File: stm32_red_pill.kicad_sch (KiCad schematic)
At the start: 29 parts, among them J1 USB_B_Micro, J2 Conn_01x18, J3 Conn_01x18, SW1 SW_SPDT, U1 STM32F103C8T6, U2 AMS1117-3.3, Y1 16MHZ

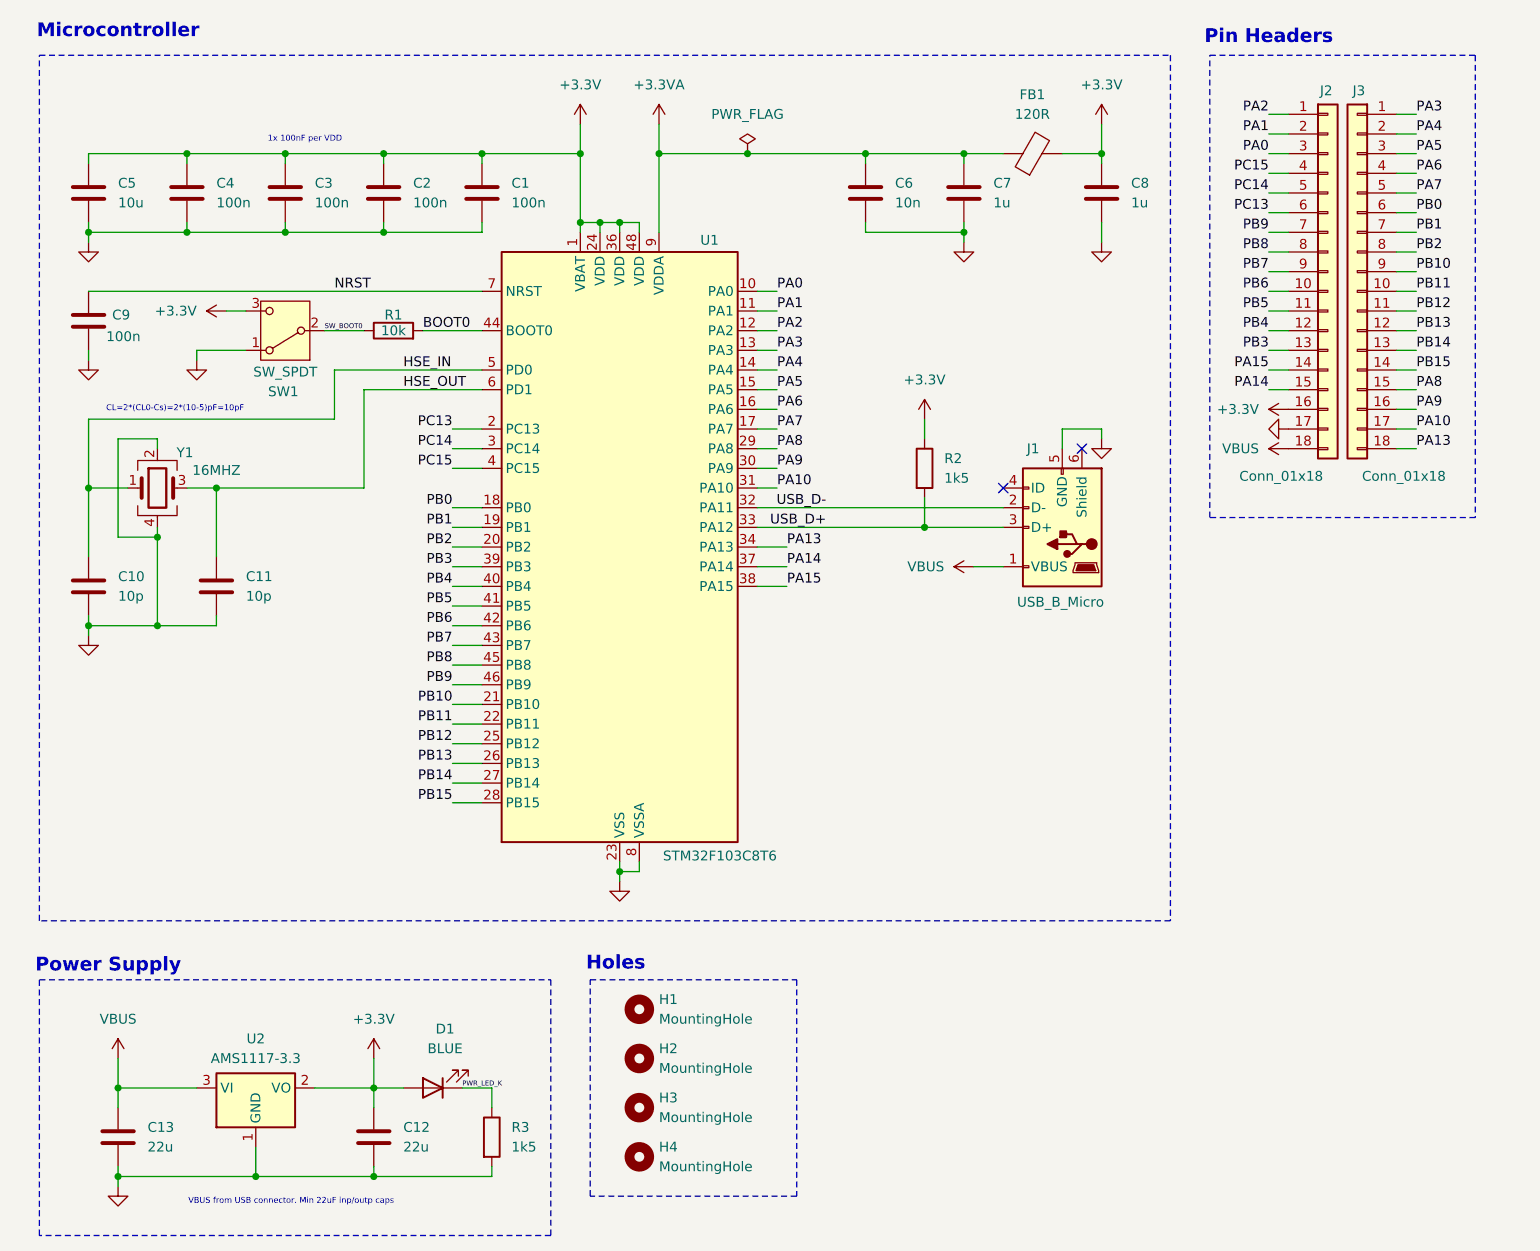
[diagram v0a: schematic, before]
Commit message: update
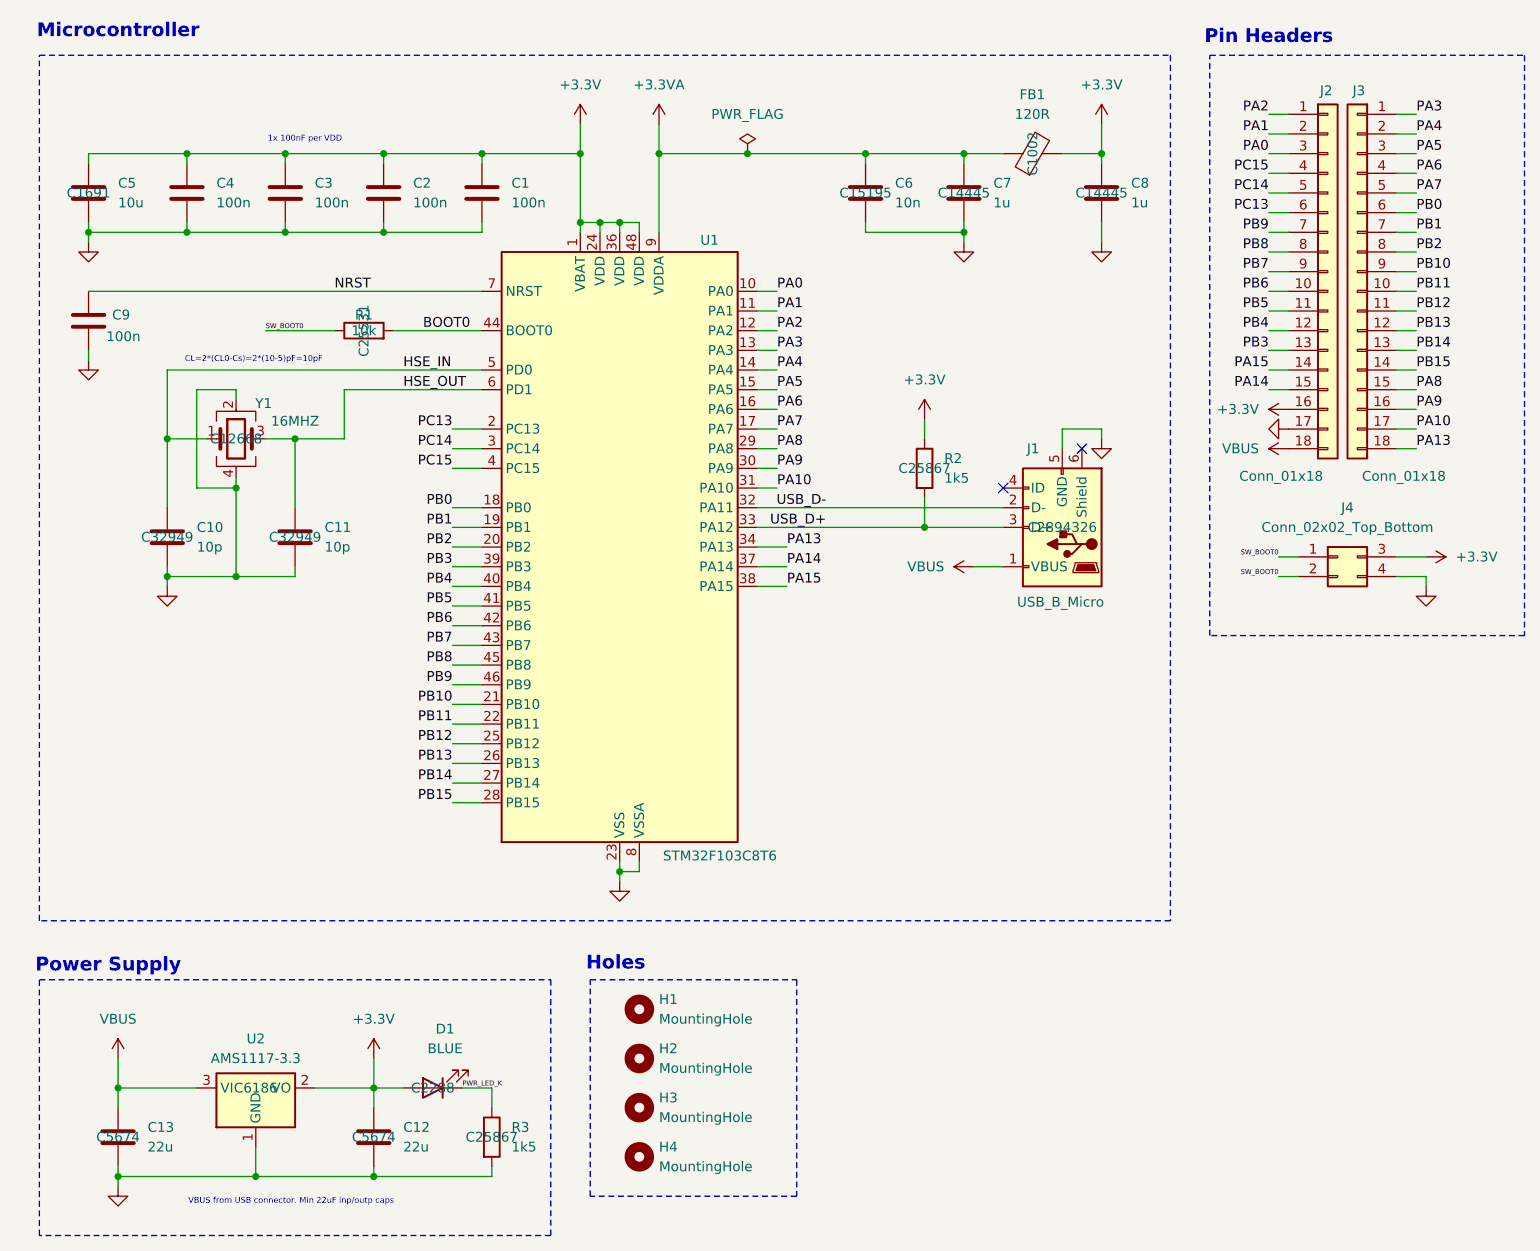
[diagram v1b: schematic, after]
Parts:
- removed SW1: SW_SPDT, Button_Switch_SMD:SW_SPDT_PCM12, symbol Switch:SW_SPDT
- added J4: Conn_02x02_Top_Bottom, Connector_PinHeader_2.54mm:PinHeader_2x02_P2.54mm_Vertical, symbol Connector_Generic:Conn_02x02_Top_Bottom
- C1, C2, C3, C4, C9: MPN (none) -> C1525
- C10, C11: MPN (none) -> C32949
- C12, C13: MPN (none) -> C5674
- C5: MPN (none) -> C1691
- C6: MPN (none) -> C15195
- C7, C8: MPN (none) -> C14445
- D1: MPN (none) -> C2288
- FB1: MPN (none) -> C1002
- J1: MPN (none) -> C2894326
- R1: MPN (none) -> C25531
- R2, R3: MPN (none) -> C25867
- U1: MPN (none) -> C8734
- U2: MPN (none) -> C6186
- Y1: MPN (none) -> C12668
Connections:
- net +3.3V: now also J4.3 (Pin_3)
- net GND: now also J4.4 (Pin_4)
- net SW_BOOT0: now also J4.1 (Pin_1), J4.2 (Pin_2)
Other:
- moved on the sheet: C10, C11, R1, Y1

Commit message: lol
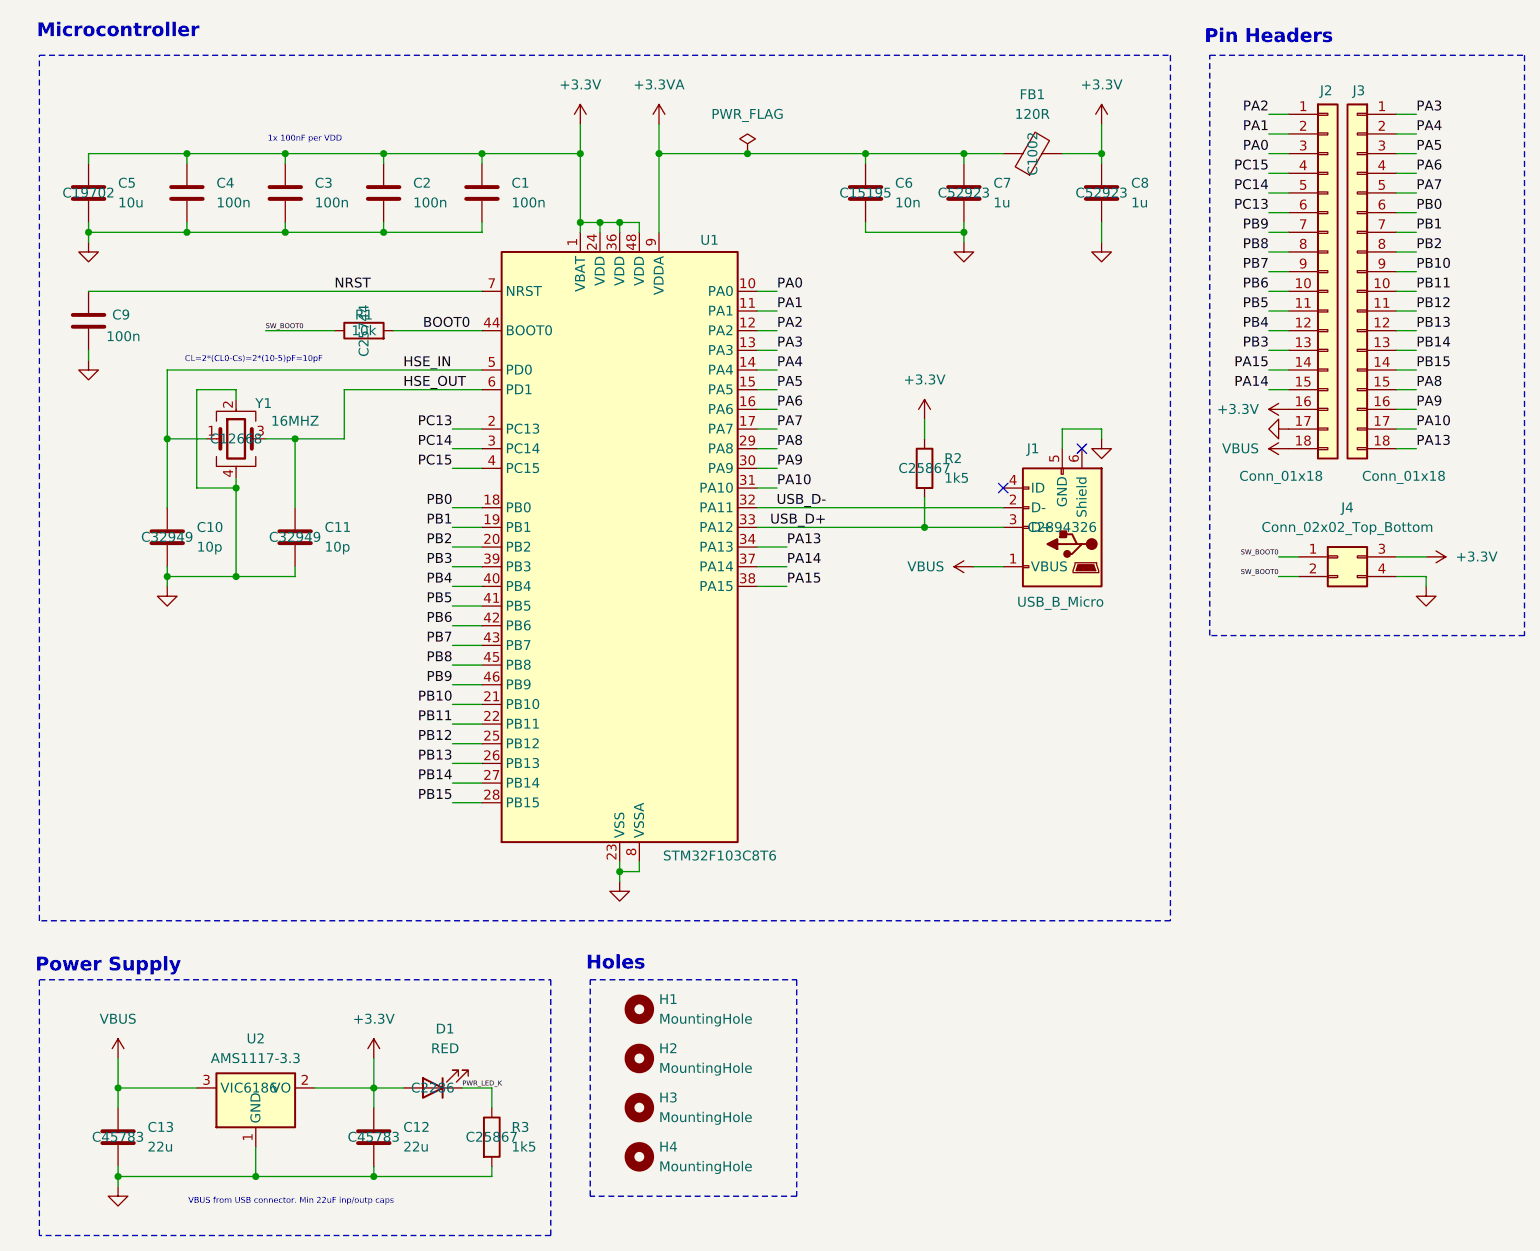
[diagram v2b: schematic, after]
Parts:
- C12, C13: MPN C5674 -> C45783
- C5: MPN C1691 -> C19702
- C7, C8: MPN C14445 -> C52923
- D1: value BLUE -> RED; MPN C2288 -> C2286
- R1: MPN C25531 -> C25744
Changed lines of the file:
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@@
 			)
 		)
-		(property "MPN" "C5674"
+		(property "MPN" "C45783"
 			(at 71.12 163.83 0)
 			(effects
@@
 			)
 		)
-		(property "MPN" "C5674"
+		(property "MPN" "C45783"
 			(at 38.1 163.83 0)
 			(effects
@@
 			)
 		)
-		(property "MPN" "C14445"
+		(property "MPN" "C52923"
 			(at 147.32 41.91 0)
 			(effects
@@
 			)
 		)
-		(property "Value" "BLUE"
+		(property "Value" "RED"
 			(at 80.3275 152.4 0)
 			(effects
@@
 			)
 		)
-		(property "MPN" "C2288"
+		(property "MPN" "C2286"
 			(at 78.74 157.48 0)
 			(effects
@@
 			)
 		)
-		(property "MPN" "C25531"
+		(property "MPN" "C25744"
 			(at 69.85 59.69 0)
 			(effects
@@
 			)
 		)
-		(property "MPN" "C1691"
+		(property "MPN" "C19702"
 			(at 34.29 41.91 0)
 			(effects
@@
 			)
 		)
-		(property "MPN" "C14445"
+		(property "MPN" "C52923"
 			(at 165.1 41.91 0)
 			(effects
